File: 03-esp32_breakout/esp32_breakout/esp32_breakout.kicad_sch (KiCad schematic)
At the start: 43 parts, among them J1 USB4110-GF-A, SW1 SW_Push, SW2 SW_Push, SW3 SW_Push, U1 ESP32-S3, U3 AP2112H, Y1 ECS-400-10-37B2-CKY-TR, Y2 ECS-.327-12.5-34B-TR

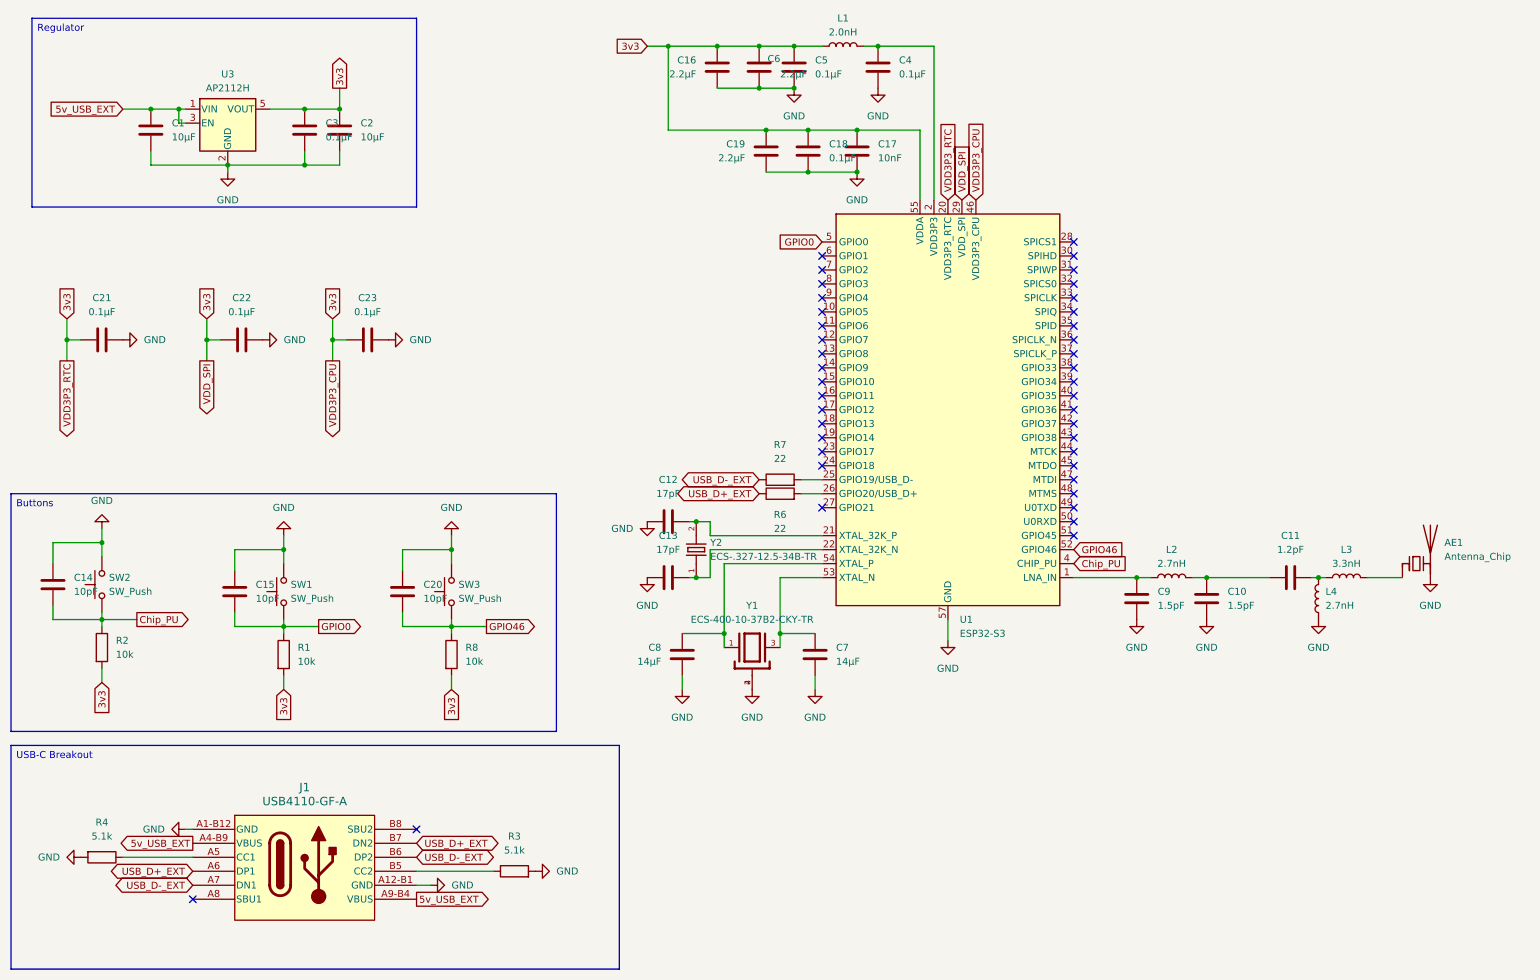
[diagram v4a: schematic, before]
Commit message: layout updates
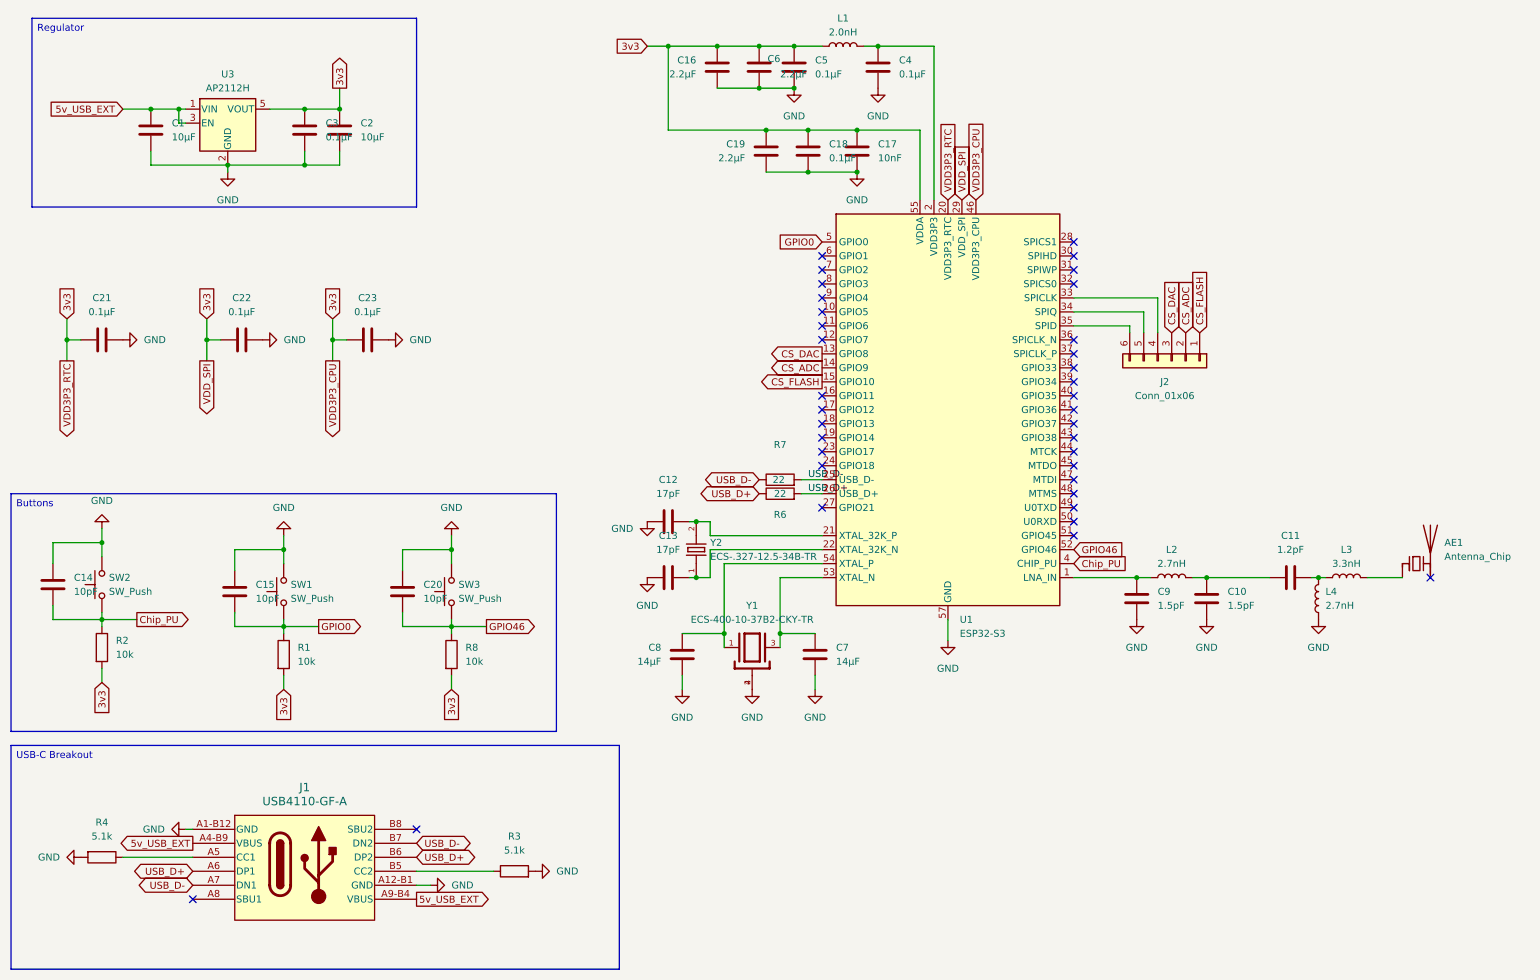
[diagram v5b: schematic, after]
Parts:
- added J2: Conn_01x06, Connector_PinHeader_1.27mm:PinHeader_1x06_P1.27mm_Vertical, symbol Connector_Generic:Conn_01x06
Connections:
- net GND: now also C7.2; no longer AE1.2 (PCB_Trace), C7.1
- net CS_DAC: now reaches U1.13 (GPIO8)
- net CS_DAC: now also J2.3 (Pin_3)
- net CS_ADC: now reaches U1.14 (GPIO9)
- net CS_ADC: now also J2.2 (Pin_2)
- net CS_FLASH: now reaches U1.15 (GPIO10)
- net CS_FLASH: now also J2.1 (Pin_1)
- net USB_D-: now reaches R7.2, U1.25 (USB_D-)
- net USB_D-: now also J1.A7 (DN1), J1.B7 (DN2), R7.1
- net USB_D+: now reaches R6.2, U1.26 (USB_D+)
- net USB_D+: now also J1.A6 (DP1), J1.B6 (DP2), R6.1
- net at U1.33 (SPICLK): now also J2.4 (Pin_4)
- net at U1.34 (SPIQ): now also J2.5 (Pin_5)
- net at U1.35 (SPID): now also J2.6 (Pin_6)
- net at U1.53 (XTAL_N), Y1.3: now also C7.1; no longer C7.2
- removed net USB_D+_EXT: J1.A6 (DP1), J1.B7 (DN2), R6.1
- removed net USB_D-_EXT: J1.A7 (DN1), J1.B6 (DP2), R7.1
- no-connect marks 41 -> 36
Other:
- moved on the sheet: C7
